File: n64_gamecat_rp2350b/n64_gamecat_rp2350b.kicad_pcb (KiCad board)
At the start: 2 copper layers, 65 x 80.5 mm, 6 parts, among them J1 Conn_01x03_Pin, J2 Conn_01x03_Pin, J3 Conn_01x05, U4 RP235x-B

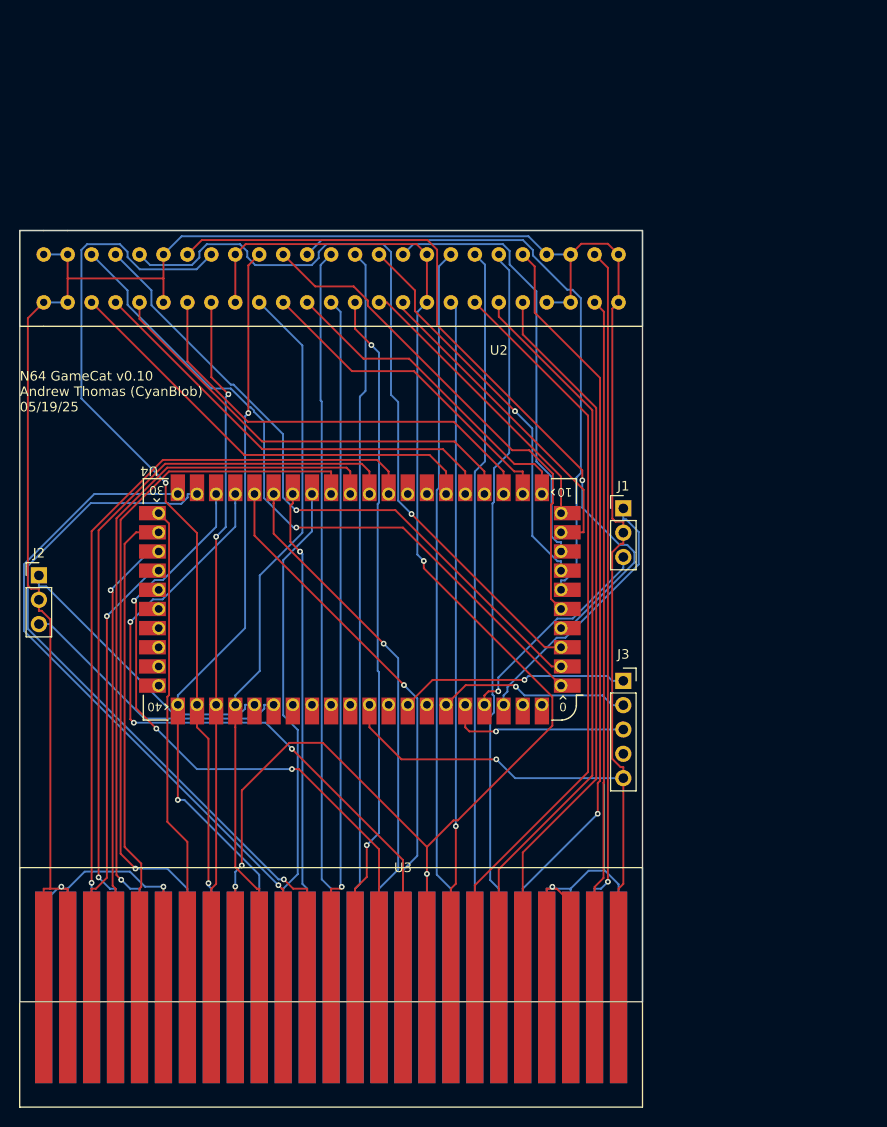
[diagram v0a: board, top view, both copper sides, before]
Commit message: Misc changes; add OoT decomp
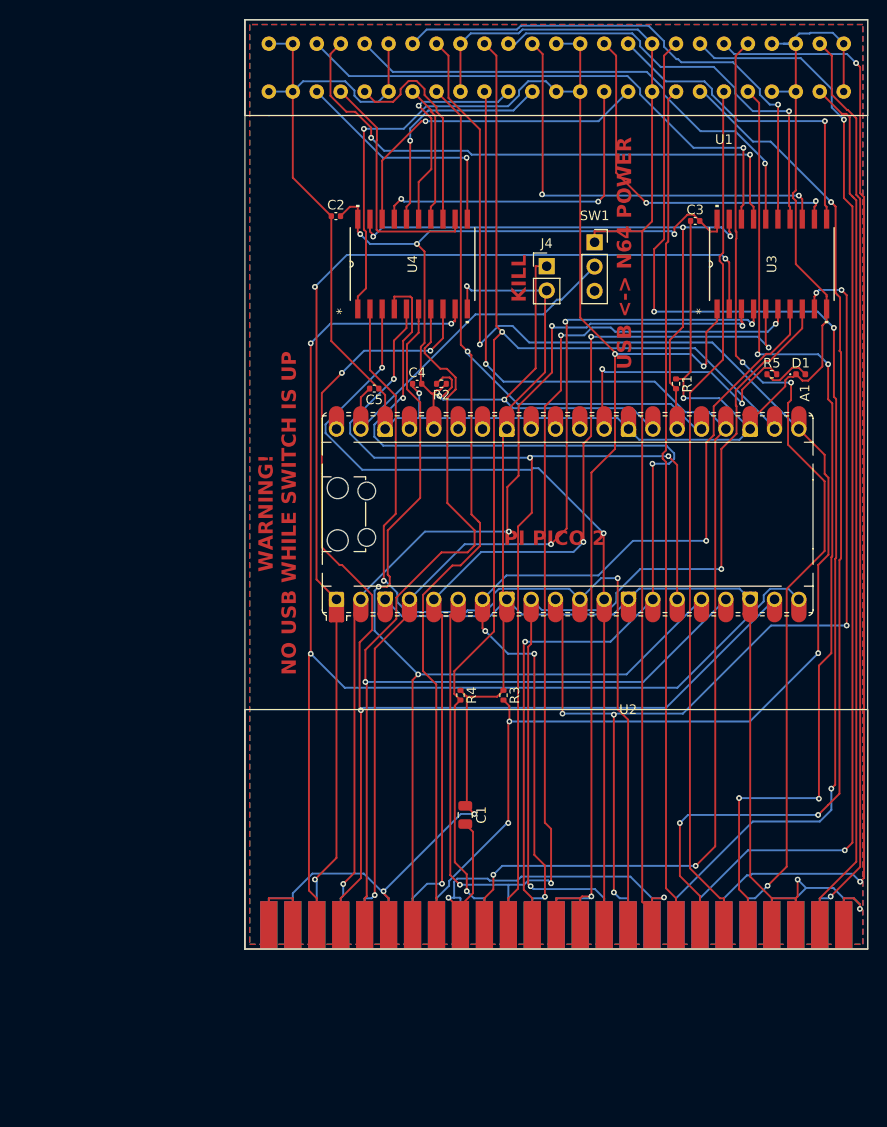
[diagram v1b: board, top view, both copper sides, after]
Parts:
- removed J1, J2: Conn_01x03_Pin, Connector_PinHeader_2.54mm:PinHeader_1x03_P2.54mm_Vertical
- removed J3: Conn_01x05, Connector_PinSocket_2.54mm:PinSocket_1x05_P2.54mm_Vertical
- added A1: RaspberryPi_Pico, Module:RaspberryPi_Pico_Common_Unspecified, F.Cu at (158.7, 93.6)
- added C1: 10uF, Capacitor_SMD:C_0805_2012Metric, F.Cu at (148.0, 125.0)
- added C2: 100nF, Capacitor_SMD:C_0402_1005Metric, F.Cu at (134.5, 62.5)
- added C3: 100nF, Capacitor_SMD:C_0402_1005Metric, F.Cu at (172.0, 63.0)
- added C4: 100nF, Capacitor_SMD:C_0402_1005Metric, F.Cu at (143.0, 80.0)
- added C5: 100nF, Capacitor_SMD:C_0402_1005Metric, F.Cu at (138.5, 80.5)
- added D1: LED, LED_SMD:LED_0402_1005Metric, F.Cu at (183.0, 79.0)
- added J4: Conn_01x02_Pin, Connector_PinHeader_2.54mm:PinHeader_1x02_P2.54mm_Vertical, F.Cu at (156.5, 67.7)
- added R1: 10K, Resistor_SMD:R_0402_1005Metric, F.Cu at (170.0, 80.0)
- added R2: 10K, Resistor_SMD:R_0402_1005Metric, F.Cu at (145.5, 80.0)
- added R3: 10K, Resistor_SMD:R_0402_1005Metric, F.Cu at (152.0, 112.5)
- added R4: 10K, Resistor_SMD:R_0402_1005Metric, F.Cu at (147.5, 112.5)
- added R5: 1K, Resistor_SMD:R_0402_1005Metric, F.Cu at (180.0, 79.0)
- added SW1: SW_SPDT, Connector_PinSocket_2.54mm:PinSocket_1x03_P2.54mm_Vertical, F.Cu at (161.5, 65.2)
- added U1: ~, n64_library:N64_cartridge_connecter_2.5mm, F.Cu at (160.0, 47.0)
- U2: footprint n64_library:N64_cartridge_connecter_2.5mm -> n64_library:N64_cartridge_pins_2.5mm
- U3: value ~ -> SN74CBTLV3245ADW; footprint n64_library:N64_cartridge_pins_2.5mm -> footprints:DW20
- U4: value RP235x-B -> SN74CBTLV3245ADW; footprint RP2xxx_Stamp:RP2xxx_Stamp_XL_THT -> footprints:DW20
- moved U3 77.2 mm to (180.0, 67.5), turned to 90 degrees
- moved U2 43.1 mm to (152.5, 109.0)
- moved U4 35.4 mm to (142.5, 67.5), turned to 90 degrees
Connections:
- U2 pad 11: CA_AD11 -> AD11
- U2 pad 12: CA_AD10 -> AD10
- U2 pad 13: Net-(U2-NC-Pad13) -> NC
- U2 pad 14: Net-(U2-NC-Pad14) -> NC
- U2 pad 15: CA_AD9 -> AD9
- U2 pad 16: CA_AD8 -> AD8
- U2 pad 17: +3V3 -> 3V3_CART
- U2 pad 18: Net-(U2-CIC_PIF) -> CIC_PIF
- U2 pad 19: Net-(U2-CLK_PIF) -> CLK_PIF
- U2 pad 20: Net-(U2-COLD_RST) -> COLD_RST
- U2 pad 21: Net-(U2-S_DAT) -> S_DAT
- U2 pad 24: Net-(U2-LAUDIO) -> LAUDIO
- U2 pad 28: CA_AD0 -> AD0
- U2 pad 29: CA_AD1 -> AD1
- U2 pad 3: CA_AD15 -> AD15
- U2 pad 30: CA_AD2 -> AD2
- U2 pad 32: CA_AD3 -> AD3
- U2 pad 34: +3V3 -> 3V3_CART
- U2 pad 36: CA_AD4 -> AD4
- U2 pad 37: CA_AD5 -> AD5
- U2 pad 38: Net-(U2-NC-Pad38) -> NC
- U2 pad 39: Net-(U2-NC-Pad39) -> NC
- U2 pad 4: CA_AD14 -> AD14
- U2 pad 40: CA_AD6 -> AD6
- U2 pad 41: CA_AD7 -> AD7
- U2 pad 42: +3V3 -> 3V3_CART
- U2 pad 43: Net-(U2-PIF_CIC) -> PIF_CIC
- U2 pad 44: Net-(U2-JTAG_CLK) -> JTAG_CLK
- U2 pad 45: Net-(U2-NMI_R4300) -> NMI_R4300
- U2 pad 46: Net-(U2-VIDEO_CLK) -> VIDEO_CLK
- U2 pad 49: Net-(U2-R_AUDIO) -> R_AUDIO
- U2 pad 5: CA_AD13 -> AD13
- U2 pad 7: CA_AD12 -> AD12
- U2 pad 9: +3V3 -> 3V3_CART
- U3 pad 1: GND -> NC
- U3 pad 10: READ -> GND
- U3 pad 11: CO_AD11 -> CA_AD7
- U3 pad 12: CO_AD10 -> CA_AD6
- U3 pad 13: Net-(U2-NC-Pad13) -> CA_AD5
- U3 pad 14: Net-(U2-NC-Pad14) -> CA_AD4
- U3 pad 15: CO_AD9 -> CA_AD3
- U3 pad 16: CO_AD8 -> CA_AD2
- U3 pad 17: +3V3 -> CA_AD1
- U3 pad 18: Net-(U2-CIC_PIF) -> CA_AD0
- U3 pad 19: Net-(U2-CLK_PIF) -> CART_EN
- U3 pad 2: GND -> AD0
- U3 pad 20: Net-(U2-COLD_RST) -> 3V3_OUT
- U3 pad 3: CO_AD15 -> AD1
- U3 pad 4: CO_AD14 -> AD2
- U3 pad 5: CO_AD13 -> AD3
- U3 pad 6: GND -> AD4
- U3 pad 7: CO_AD12 -> AD5
- U3 pad 8: WRITE -> AD6
- U3 pad 9: +3V3 -> AD7
- U4 pad 1: CA_AD0 -> NC
- U4 pad 10: CA_AD9 -> GND
- U4 pad 11: CA_AD10 -> CA_AD15
- U4 pad 12: CA_AD11 -> CA_AD14
- U4 pad 13: CA_AD12 -> CA_AD13
- U4 pad 14: CA_AD13 -> CA_AD12
- U4 pad 15: CA_AD14 -> CA_AD11
- U4 pad 16: CA_AD15 -> CA_AD10
- U4 pad 17: unconnected-(U4-GPIO16-Pad17) -> CA_AD9
- U4 pad 18: unconnected-(U4-GPIO17-Pad18) -> CA_AD8
- U4 pad 19: CO_AD0 -> CART_EN
- U4 pad 2: CA_AD1 -> AD8
- U4 pad 20: CO_AD1 -> 3V3_OUT
- U4 pad 3: CA_AD2 -> AD9
- U4 pad 4: CA_AD3 -> AD10
- U4 pad 5: CA_AD4 -> AD11
- U4 pad 6: CA_AD5 -> AD12
- U4 pad 7: CA_AD6 -> AD13
- U4 pad 8: CA_AD7 -> AD14
- U4 pad 9: CA_AD8 -> AD15
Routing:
- net +3V3: track 183.4 -> 0.00 mm, vias 4 -> 0
- net NC: track 0.00 -> 173.7 mm, vias 0 -> 4
- net 3V3_CART: track 0.00 -> 169.5 mm, vias 0 -> 2
- net AD15: track 0.00 -> 136.0 mm, vias 0 -> 3
- net AD4: track 0.00 -> 126.9 mm, vias 0 -> 4
- net AD14: track 0.00 -> 125.4 mm, vias 0 -> 3
- net PIF_CIC: track 0.00 -> 121.8 mm, vias 0 -> 3
- net NMI_R4300: track 0.00 -> 119.0 mm, vias 0 -> 2
- net AD0: track 0.00 -> 117.6 mm, vias 0 -> 3
- net JTAG_CLK: track 0.00 -> 116.4 mm, vias 0 -> 2
- net AD13: track 0.00 -> 115.5 mm, vias 0 -> 1
- net AD11: track 0.00 -> 115.0 mm, vias 0 -> 3
- net AD10: track 0.00 -> 113.8 mm, vias 0 -> 3
- net CLK_PIF: track 0.00 -> 109.9 mm, vias 0 -> 3
- net AD7: track 0.00 -> 107.9 mm, vias 0 -> 6
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- added copper zone on B.Cu, net GND
- added copper zone on F.Cu, net GND
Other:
- board size 65 x 80.5 mm -> 65 x 97 mm
- board text added: "KILL"
- board text added: "PI PICO 2"
- board text added: "USB <-> N64 POWER"
- board text added: "WARNING! NO USB WHILE SWITCH IS UP"
- board text removed: "N64 GameCat v0.10 Andrew Thomas (CyanBlob) 05/19/25"
